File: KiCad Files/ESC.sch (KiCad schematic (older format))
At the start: 97 parts, among them J1 Conn_01x03, J10 Conn_01x03, J11 Conn_01x04, J2 Conn_01x06_Female, J3 Conn_01x01, J4 Conn_01x01, J5 Conn_01x01, J6 Conn_01x03, J7 Conn_01x02, J8 Conn_01x04, J9 Conn_01x03, Q1 IRF3205, Q2 IRF3205, Q3 IRF3205, Q4 IRF3205, Q5 IRF3205, Q6 IRF3205, U1 LM339, U2 L7809, U3 MCP601-xP, U4 IR2110, U5 IR2110, U6 IR2110

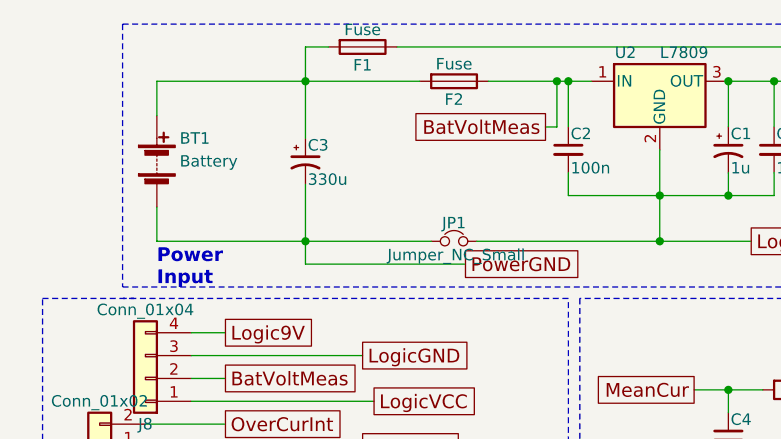
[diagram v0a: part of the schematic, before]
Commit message: Added final PCB
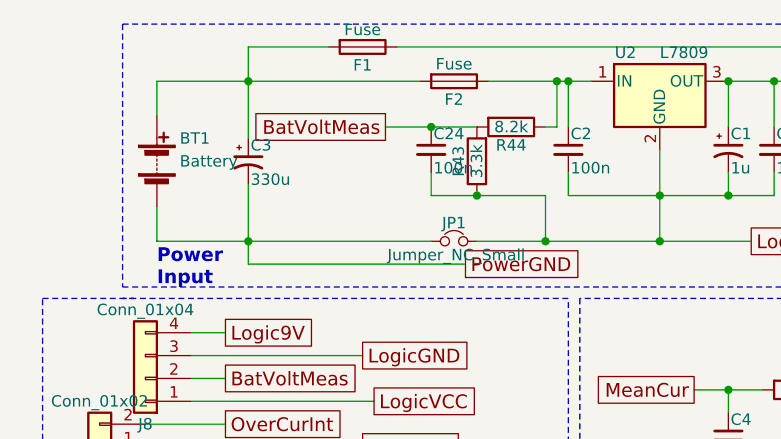
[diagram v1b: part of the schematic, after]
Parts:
- added C24: 100n, Capacitors_SMD:C_1206_HandSoldering, symbol C_Small
- added R43: 3.3k, Resistors_SMD:R_1206_HandSoldering, symbol R
- added R44: 8.2k, Resistors_SMD:R_1206_HandSoldering, symbol R
- C10, C9: footprint Capacitors_THT:C_Disc_D8.0mm_W5.0mm_P5.00mm -> Capacitors_SMD:C_1206_HandSoldering
- C11: footprint Capacitors_THT:C_Disc_D8.0mm_W2.5mm_P5.00mm -> Capacitors_SMD:C_1206_HandSoldering
- C12, C13, C14: footprint Capacitors_THT:C_Disc_D7.5mm_W5.0mm_P5.00mm -> Capacitors_SMD:C_1206_HandSoldering
- C15, C16, C17, C4, C5, C6, C7, C8: footprint Capacitors_THT:C_Disc_D3.0mm_W1.6mm_P2.50mm -> Capacitors_SMD:C_1206_HandSoldering
- C18, C19, C20: footprint Capacitors_THT:C_Disc_D4.3mm_W1.9mm_P5.00mm -> Capacitors_SMD:C_1206_HandSoldering
- C2: footprint Capacitors_THT:C_Rect_L7.0mm_W2.5mm_P5.00mm -> Capacitors_SMD:C_1206_HandSoldering
- C21, C22, C23: footprint Capacitors_THT:C_Rect_L7.2mm_W11.0mm_P5.00mm_FKS2_FKP2_MKS2_MKP2 -> Capacitors_THT:C_Disc_D4.3mm_W1.9mm_P5.00mm
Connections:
- net BatVoltMeas: now also C24.1, R43.2, R44.2; no longer C2.1, F2.1, U2.1 (IN)
- net LogicGND: now also C24.2, R43.1
- new net: C2.1, F2.1, R44.1, U2.1 (IN)
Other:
- moved on the sheet: C3
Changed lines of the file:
@@
 F 0 "C18" H 8160 1470 50  0000 L CNN
 F 1 "1u" H 8160 1320 50  0000 L CNN
-F 2 "Capacitors_THT:C_Disc_D4.3mm_W1.9mm_P5.00mm" H 8150 1400 50  0001 C CNN
+F 2 "Capacitors_SMD:C_1206_HandSoldering" H 8150 1400 50  0001 C CNN
 F 3 "" H 8150 1400 50  0001 C CNN
 	1    8150 1400
@@
 F 0 "C15" H 7960 1970 50  0000 L CNN
 F 1 "33n" H 7960 1820 50  0000 L CNN
-F 2 "Capacitors_THT:C_Disc_D3.0mm_W1.6mm_P2.50mm" H 7950 1900 50  0001 C CNN
+F 2 "Capacitors_SMD:C_1206_HandSoldering" H 7950 1900 50  0001 C CNN
 F 3 "" H 7950 1900 50  0001 C CNN
 	1    7950 1900
@@
 F 0 "C12" H 6910 1220 50  0000 L CNN
 F 1 "10n" H 6910 1070 50  0000 L CNN
-F 2 "Capacitors_THT:C_Disc_D7.5mm_W5.0mm_P5.00mm" H 6900 1150 50  0001 C CNN
+F 2 "Capacitors_SMD:C_1206_HandSoldering" H 6900 1150 50  0001 C CNN
 F 3 "" H 6900 1150 50  0001 C CNN
 	1    6900 1150
@@
 F 0 "C2" H 2810 1170 50  0000 L CNN
 F 1 "100n" H 2810 1020 50  0000 L CNN
-F 2 "Capacitors_THT:C_Rect_L7.0mm_W2.5mm_P5.00mm" H 2800 1100 50  0001 C CNN
+F 2 "Capacitors_SMD:C_1206_HandSoldering" H 2800 1100 50  0001 C CNN
 F 3 "" H 2800 1100 50  0001 C CNN
 	1    2800 1100
@@
 F 0 "C19" H 8160 3320 50  0000 L CNN
 F 1 "1u" H 8160 3170 50  0000 L CNN
-F 2 "Capacitors_THT:C_Disc_D4.3mm_W1.9mm_P5.00mm" H 8150 3250 50  0001 C CNN
+F 2 "Capacitors_SMD:C_1206_HandSoldering" H 8150 3250 50  0001 C CNN
 F 3 "" H 8150 3250 50  0001 C CNN
 	1    8150 3250
@@
 F 0 "C16" H 7960 3820 50  0000 L CNN
 F 1 "33n" H 7960 3670 50  0000 L CNN
-F 2 "Capacitors_THT:C_Disc_D3.0mm_W1.6mm_P2.50mm" H 7950 3750 50  0001 C CNN
+F 2 "Capacitors_SMD:C_1206_HandSoldering" H 7950 3750 50  0001 C CNN
 F 3 "" H 7950 3750 50  0001 C CNN
 	1    7950 3750
@@
 F 0 "C13" H 6910 3070 50  0000 L CNN
 F 1 "10n" H 6910 2920 50  0000 L CNN
-F 2 "Capacitors_THT:C_Disc_D7.5mm_W5.0mm_P5.00mm" H 6900 3000 50  0001 C CNN
+F 2 "Capacitors_SMD:C_1206_HandSoldering" H 6900 3000 50  0001 C CNN
 F 3 "" H 6900 3000 50  0001 C CNN
 	1    6900 3000
@@
 F 0 "C20" H 8160 5170 50  0000 L CNN
 F 1 "1u" H 8160 5020 50  0000 L CNN
-F 2 "Capacitors_THT:C_Disc_D4.3mm_W1.9mm_P5.00mm" H 8150 5100 50  0001 C CNN
+F 2 "Capacitors_SMD:C_1206_HandSoldering" H 8150 5100 50  0001 C CNN
 F 3 "" H 8150 5100 50  0001 C CNN
 	1    8150 5100
@@
 F 0 "C17" H 7960 5670 50  0000 L CNN
 F 1 "33n" H 7960 5520 50  0000 L CNN
-F 2 "Capacitors_THT:C_Disc_D3.0mm_W1.6mm_P2.50mm" H 7950 5600 50  0001 C CNN
+F 2 "Capacitors_SMD:C_1206_HandSoldering" H 7950 5600 50  0001 C CNN
 F 3 "" H 7950 5600 50  0001 C CNN
 	1    7950 5600
@@
 F 0 "C14" H 6910 4920 50  0000 L CNN
 F 1 "10n" H 6910 4770 50  0000 L CNN
-F 2 "Capacitors_THT:C_Disc_D7.5mm_W5.0mm_P5.00mm" H 6900 4850 50  0001 C CNN
+F 2 "Capacitors_SMD:C_1206_HandSoldering" H 6900 4850 50  0001 C CNN
 F 3 "" H 6900 4850 50  0001 C CNN
 	1    6900 4850
@@
 F 0 "C11" H 6310 7470 50  0000 L CNN
 F 1 "6.8n" H 6310 7320 50  0000 L CNN
-F 2 "Capacitors_THT:C_Disc_D8.0mm_W2.5mm_P5.00mm" H 6300 7400 50  0001 C CNN
+F 2 "Capacitors_SMD:C_1206_HandSoldering" H 6300 7400 50  0001 C CNN
 F 3 "" H 6300 7400 50  0001 C CNN
 	1    6300 7400
@@
 F 0 "C8" H 4210 7120 50  0000 L CNN
 F 1 "1n" H 4210 6970 50  0000 L CNN
-F 2 "Capacitors_THT:C_Disc_D3.0mm_W1.6mm_P2.50mm" H 4200 7050 50  0001 C CNN
+F 2 "Capacitors_SMD:C_1206_HandSoldering" H 4200 7050 50  0001 C CNN
 F 3 "" H 4200 7050 50  0001 C CNN
 	1    4200 7050
@@
 F 0 "C7" H 3860 7120 50  0000 L CNN
 F 1 "1n" H 3860 6970 50  0000 L CNN
-F 2 "Capacitors_THT:C_Disc_D3.0mm_W1.6mm_P2.50mm" H 3850 7050 50  0001 C CNN
+F 2 "Capacitors_SMD:C_1206_HandSoldering" H 3850 7050 50  0001 C CNN
 F 3 "" H 3850 7050 50  0001 C CNN
 	1    3850 7050
@@
 F 0 "C5" H 3510 7120 50  0000 L CNN
 F 1 "1n" H 3510 6970 50  0000 L CNN
-F 2 "Capacitors_THT:C_Disc_D3.0mm_W1.6mm_P2.50mm" H 3500 7050 50  0001 C CNN
+F 2 "Capacitors_SMD:C_1206_HandSoldering" H 3500 7050 50  0001 C CNN
 F 3 "" H 3500 7050 50  0001 C CNN
 	1    3500 7050
@@
 F 0 "C9" H 4610 1220 50  0000 R CNN
 F 1 "5.6n" H 4610 1070 50  0000 R CNN
-F 2 "Capacitors_THT:C_Disc_D8.0mm_W5.0mm_P5.00mm" H 4600 1150 50  0001 C CNN
+F 2 "Capacitors_SMD:C_1206_HandSoldering" H 4600 1150 50  0001 C CNN
 F 3 "" H 4600 1150 50  0001 C CNN
 	1    4600 1150
@@
 F 0 "C10" H 5760 1770 50  0000 L CNN
 F 1 "5.6n" H 5760 1620 50  0000 L CNN
-F 2 "Capacitors_THT:C_Disc_D8.0mm_W5.0mm_P5.00mm" H 5750 1700 50  0001 C CNN
+F 2 "Capacitors_SMD:C_1206_HandSoldering" H 5750 1700 50  0001 C CNN
 F 3 "" H 5750 1700 50  0001 C CNN
 	1    5750 1700
@@
 Text GLabel 3350 2150 0    60   UnSpc ~ 0
 MeanCur
-Text GLabel 2700 1000 0    60   UnSpc ~ 0
+Text GLabel 2000 1000 0    60   UnSpc ~ 0
 BatVoltMeas
 Text Notes 2950 3500 0    60   ~ 12
@@
 F 0 "C4" H 3510 2420 50  0000 L CNN
 F 1 "33n" H 3510 2270 50  0000 L CNN
-F 2 "Capacitors_THT:C_Disc_D3.0mm_W1.6mm_P2.50mm" H 3500 2350 50  0001 C CNN
+F 2 "Capacitors_SMD:C_1206_HandSoldering" H 3500 2350 50  0001 C CNN
 F 3 "" H 3500 2350 50  0001 C CNN
 	1    3500 2350
@@
 F 0 "C6" H 3710 1170 50  0000 L CNN
 F 1 "1n" H 3710 1020 50  0000 L CNN
-F 2 "Capacitors_THT:C_Disc_D3.0mm_W1.6mm_P2.50mm" H 3700 1100 50  0001 C CNN
+F 2 "Capacitors_SMD:C_1206_HandSoldering" H 3700 1100 50  0001 C CNN
 F 3 "" H 3700 1100 50  0001 C CNN
 	1    3700 1100
@@
 	8300 750  9550 750
 Wire Wire Line
-	1650 1600 2350 1600
-Connection ~ 1650 1500
+	1400 1600 2350 1600
 Wire Wire Line
 	1000 1350 1000 1500
-Connection ~ 1650 800
-Wire Wire Line
-	1650 650  1650 1050
 Wire Wire Line
 	7350 2050 7350 1950
@@
 Connection ~ 9400 1500
 Wire Wire Line
-	1650 650  1750 650
+	1400 650  1750 650
 Wire Wire Line
 	2050 650  4900 650
@@
 Wire Notes Line
 	6050 550  4200 550
-Wire Wire Line
-	1650 1250 1650 1600
 Wire Wire Line
 	950  2400 1900 2400
@@
 L CP1_Small C3
 U 1 1 5ACE5B95
-P 1650 1150
-F 0 "C3" H 1660 1220 50  0000 L CNN
-F 1 "330u" H 1660 1070 50  0000 L CNN
-F 2 "Capacitors_THT:CP_Radial_D12.5mm_P7.50mm" H 1650 1150 50  0001 C CNN
-F 3 "" H 1650 1150 50  0001 C CNN
-	1    1650 1150
+P 1400 1150
+F 0 "C3" H 1410 1220 50  0000 L CNN
+F 1 "330u" H 1410 1070 50  0000 L CNN
+F 2 "Capacitors_THT:CP_Radial_D12.5mm_P7.50mm" H 1400 1150 50  0001 C CNN
+F 3 "" H 1400 1150 50  0001 C CNN
+	1    1400 1150
 	1    0    0    -1
 $EndComp
@@
 F 0 "C21" H 9810 1320 50  0000 L CNN
 F 1 "1u" H 9810 1170 50  0000 L CNN
-F 2 "Capacitors_THT:C_Rect_L7.2mm_W11.0mm_P5.00mm_FKS2_FKP2_MKS2_MKP2" H 9800 1250 50  0001 C CNN
+F 2 "Capacitors_THT:C_Disc_D4.3mm_W1.9mm_P5.00mm" H 9800 1250 50  0001 C CNN
 F 3 "" H 9800 1250 50  0001 C CNN
 	1    9800 1250
@@
 F 0 "C22" H 9810 3170 50  0000 L CNN
 F 1 "1u" H 9810 3020 50  0000 L CNN
-F 2 "Capacitors_THT:C_Rect_L7.2mm_W11.0mm_P5.00mm_FKS2_FKP2_MKS2_MKP2" H 9800 3100 50  0001 C CNN
+F 2 "Capacitors_THT:C_Disc_D4.3mm_W1.9mm_P5.00mm" H 9800 3100 50  0001 C CNN
 F 3 "" H 9800 3100 50  0001 C CNN
 	1    9800 3100
@@
 F 0 "C23" H 9810 5020 50  0000 L CNN
 F 1 "1u" H 9810 4870 50  0000 L CNN
-F 2 "Capacitors_THT:C_Rect_L7.2mm_W11.0mm_P5.00mm_FKS2_FKP2_MKS2_MKP2" H 9800 4950 50  0001 C CNN
+F 2 "Capacitors_THT:C_Disc_D4.3mm_W1.9mm_P5.00mm" H 9800 4950 50  0001 C CNN
 F 3 "" H 9800 4950 50  0001 C CNN
 	1    9800 4950
@@
 Wire Notes Line
 	500  1750 900  1750
+Wire Wire Line
+	1400 1600 1400 1250
+Connection ~ 1400 1500
+Wire Wire Line
+	1400 650  1400 1050
+Connection ~ 1400 800
+$Comp
+L R R44
+U 1 1 5AF5E6D9
+P 2550 1000
+F 0 "R44" V 2630 1000 50  0000 C CNN
+F 1 "8.2k" V 2550 1000 50  0000 C CNN
+F 2 "Resistors_SMD:R_1206_HandSoldering" V 2480 1000 50  0001 C CNN
+F 3 "" H 2550 1000 50  0001 C CNN
+	1    2550 1000
+	0    1    1    0
+$EndComp
+$Comp
+L R R43
+U 1 1 5AF5E968
+P 2400 1150
+F 0 "R43" V 2480 1150 50  0000 C CNN
+F 1 "3.3k" V 2400 1150 50  0000 C CNN
+F 2 "Resistors_SMD:R_1206_HandSoldering" V 2330 1150 50  0001 C CNN
+F 3 "" H 2400 1150 50  0001 C CNN
+	1    2400 1150
+	-1   0    0    1
+$EndComp
+$Comp
+L C_Small C24
+U 1 1 5AF5EAE3
+P 2200 1100
+F 0 "C24" H 2210 1170 50  0000 L CNN
+F 1 "100n" H 2210 1020 50  0000 L CNN
+F 2 "Capacitors_SMD:C_1206_HandSoldering" H 2200 1100 50  0001 C CNN
+F 3 "" H 2200 1100 50  0001 C CNN
+	1    2200 1100
+	1    0    0    -1
+$EndComp
+Wire Wire Line
+	2200 1300 2200 1200
+Wire Wire Line
+	2000 1000 2400 1000
+Connection ~ 2200 1000
+Wire Wire Line
+	2200 1300 2700 1300
+Wire Wire Line
+	2700 1300 2700 1500
+Connection ~ 2700 1500
+Connection ~ 2400 1300
 $EndSCHEMATC
